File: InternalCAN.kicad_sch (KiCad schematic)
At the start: 8 parts, among them IC3 TCAN337DCNR, U4 CDSOT23-T24CAN

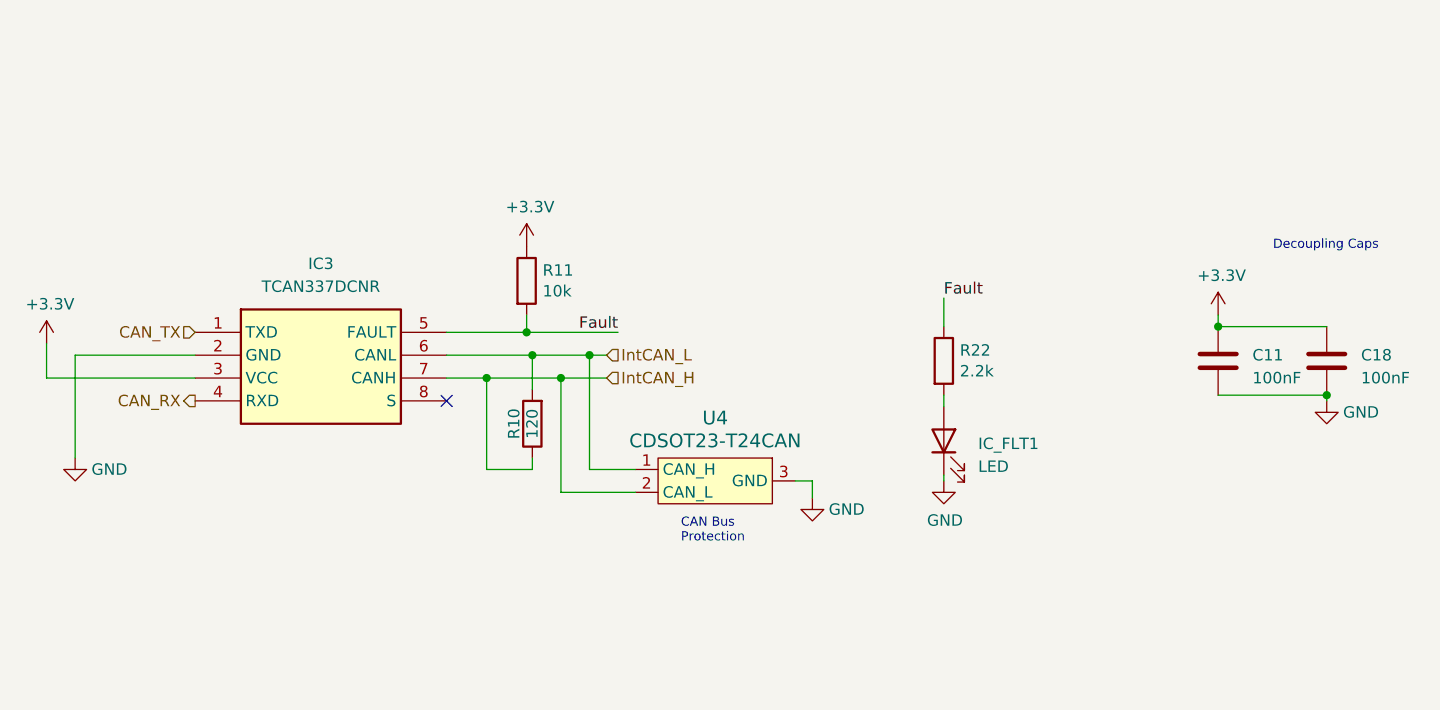
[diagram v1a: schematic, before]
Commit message: MCU pins, PSON power distribution, KiCad-Sharepoint, and 7 seg
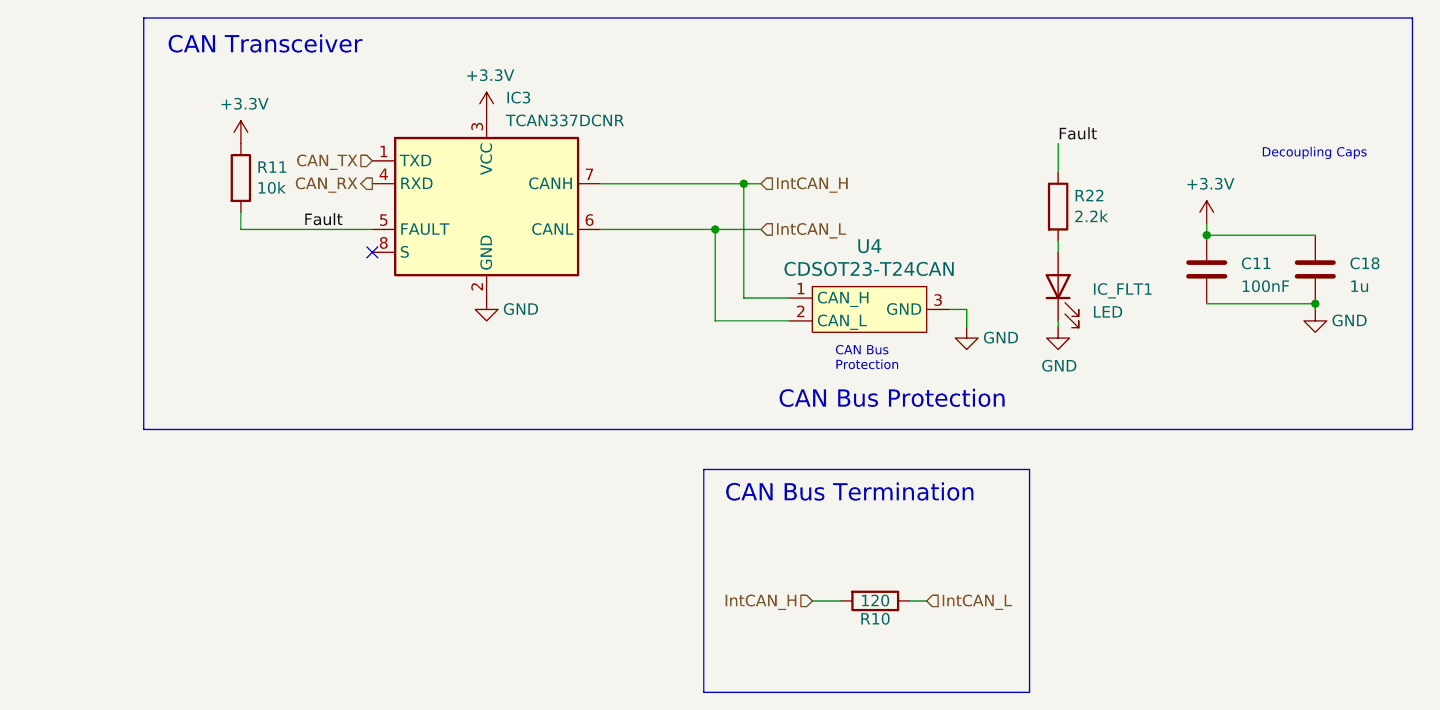
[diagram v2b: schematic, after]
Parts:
- C18: value 100nF -> 1u
- IC3: footprint UTSVT_ICs:SOT65P280X145-8N -> UTSVT_ICs:TCAN337DCNR; symbol utsvt-chips:TCAN337DCNR -> UTSVT-ICs:TCAN337; P/N (none) -> TCAN337DCNR
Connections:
- net IntCAN_H: now also R10.2, U4.1 (CAN_H); no longer R10.1, U4.2 (CAN_L)
- net IntCAN_L: now also R10.1, U4.2 (CAN_L); no longer R10.2, U4.1 (CAN_H)
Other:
- note added: "CAN Bus Termination"
- note added: "CAN Transceiver"
- moved on the sheet: C11, C18, IC3, IC_FLT1, R10, R11, R22, U4
